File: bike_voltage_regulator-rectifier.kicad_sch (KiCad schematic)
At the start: 25 parts, among them U1 GBU1510_C22447862, U2 IRFB4110PBF, U3 MBR2045CT_C173461, U4 LM2903DRG4, U5 TL431_C181103, U6 MMBT3904, U7 MMBT3906LT1G, U8 436500400

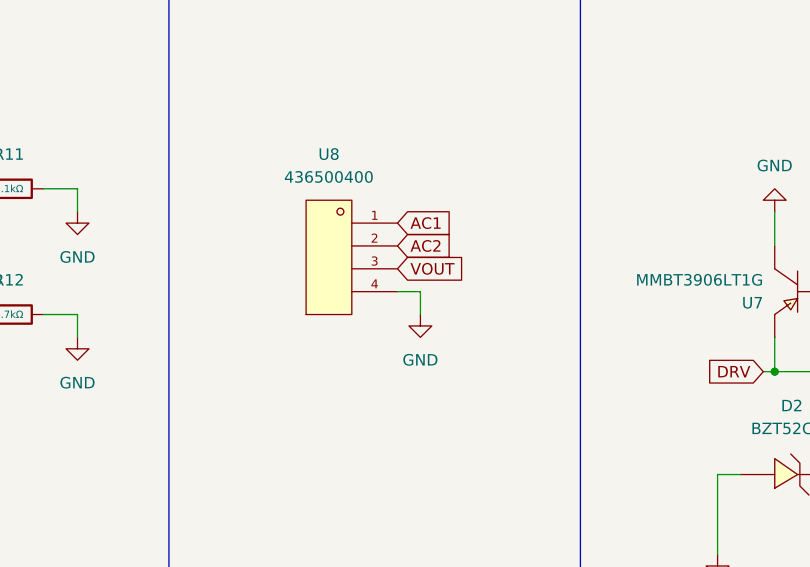
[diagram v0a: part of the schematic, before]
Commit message: first prototype
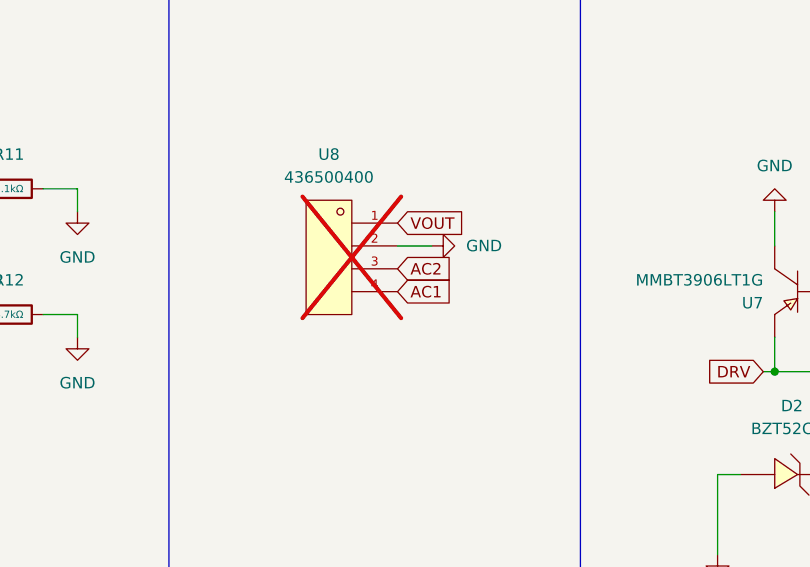
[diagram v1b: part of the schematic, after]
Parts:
- U8: now not fitted; now left out of the parts list
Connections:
- net AC1: now also U8.4; no longer U8.1
- net AC2: now also U8.3; no longer U8.2
- net GND: now also U8.2; no longer U8.4
- net VOUT: now also U8.1; no longer U8.3
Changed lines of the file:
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@@
 	(wire
 		(pts
+			(xy 100.33 139.7) (xy 104.14 139.7)
+		)
+		(stroke
+			(width 0)
+			(type default)
+		)
+	)
+	(wire
+		(pts
 			(xy 151.13 114.3) (xy 151.13 144.78)
 		)
@@
 	(wire
 		(pts
-			(xy 100.33 144.78) (xy 102.87 144.78)
-		)
-		(stroke
-			(width 0)
-			(type default)
-		)
-	)
-	(wire
-		(pts
 			(xy 142.24 153.67) (xy 151.13 153.67)
 		)
@@
 	(wire
 		(pts
-			(xy 102.87 144.78) (xy 102.87 147.32)
-		)
-		(stroke
-			(width 0)
-			(type default)
-		)
-	)
-	(wire
-		(pts
 			(xy 168.91 119.38) (xy 171.45 119.38)
 		)
@@
 	(global_label "AC1"
 		(shape input)
-		(at 100.33 137.16 0)
+		(at 100.33 144.78 0)
 		(fields_autoplaced yes)
 		(effects
@@
 		)
 		(property "Intersheetrefs" "${INTERSHEET_REFS}"
-			(at 106.8833 137.16 0)
+			(at 106.8833 144.78 0)
 			(hide yes)
 			(show_name no)
@@
 	(global_label "AC2"
 		(shape input)
-		(at 100.33 139.7 0)
+		(at 100.33 142.24 0)
 		(fields_autoplaced yes)
 		(effects
@@
 		)
 		(property "Intersheetrefs" "${INTERSHEET_REFS}"
-			(at 106.8833 139.7 0)
+			(at 106.8833 142.24 0)
 			(hide yes)
 			(show_name no)
@@
 	(global_label "VOUT"
 		(shape input)
-		(at 100.33 142.24 0)
+		(at 100.33 137.16 0)
 		(fields_autoplaced yes)
 		(effects
@@
 		)
 		(property "Intersheetrefs" "${INTERSHEET_REFS}"
-			(at 108.0324 142.24 0)
+			(at 108.0324 137.16 0)
 			(hide yes)
 			(show_name no)
@@
 	(symbol
 		(lib_id "power:GND")
-		(at 102.87 147.32 0)
+		(at 104.14 139.7 90)
 		(unit 1)
 		(body_style 1)
@@
 		(fields_autoplaced yes)
 		(property "Reference" "#PWR017"
-			(at 102.87 153.67 0)
+			(at 110.49 139.7 0)
 			(hide yes)
 			(show_name no)
@@
 		)
 		(property "Value" "GND"
-			(at 102.87 152.4 0)
+			(at 107.95 139.6999 90)
 			(show_name no)
 			(do_not_autoplace no)
@@
 					(size 1.27 1.27)
 				)
+				(justify right)
 			)
 		)
 		(property "Footprint" ""
-			(at 102.87 147.32 0)
+			(at 104.14 139.7 0)
 			(hide yes)
 			(show_name no)
@@
 		)
 		(property "Datasheet" ""
-			(at 102.87 147.32 0)
+			(at 104.14 139.7 0)
 			(hide yes)
 			(show_name no)
@@
 		)
 		(property "Description" "Power symbol creates a global label with name \"GND\" , ground"
-			(at 102.87 147.32 0)
+			(at 104.14 139.7 0)
 			(hide yes)
 			(show_name no)
@@
 		(body_style 1)
 		(exclude_from_sim no)
-		(in_bom yes)
+		(in_bom no)
 		(on_board yes)
 		(in_pos_files yes)
-		(dnp no)
+		(dnp yes)
 		(fields_autoplaced yes)
 		(property "Reference" "U8"
